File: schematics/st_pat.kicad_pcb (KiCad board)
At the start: 2 copper layers, 121.9 x 87 mm, 21 parts, among them J4 BATTERY, SW1 SW_PWR, SW2 BTN_RST, SW3 BTN, SW4 BTN, SW5 BTN, U1 GPS_Breakout_746, U2 FEATHER_M0_BASIC_PROTO, U3 LIS2MDL_ADAFRUIT, U4 Sharp_Display_4694, U5 COTS_GPS_RECEIVER, U6 SRAD_GPS_RECEIVER

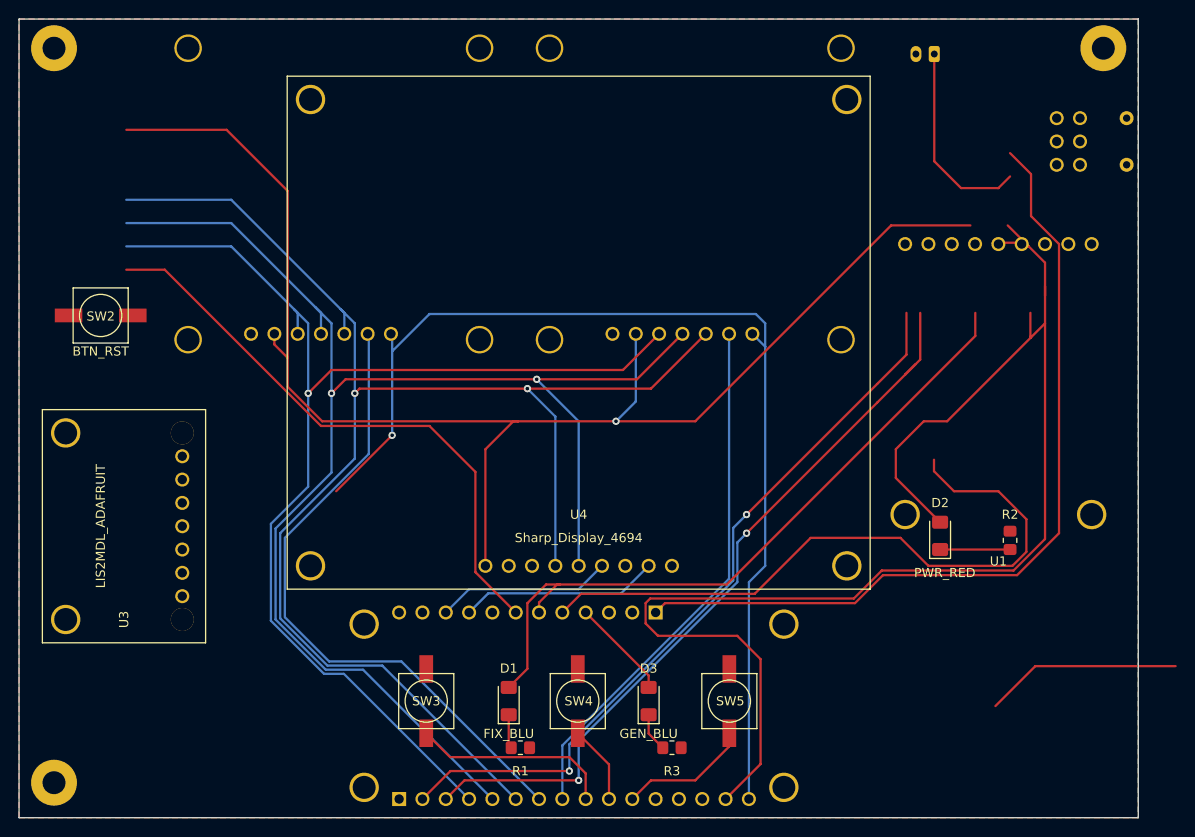
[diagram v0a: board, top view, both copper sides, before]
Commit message: wip: redo layout and use diffrent button footprint
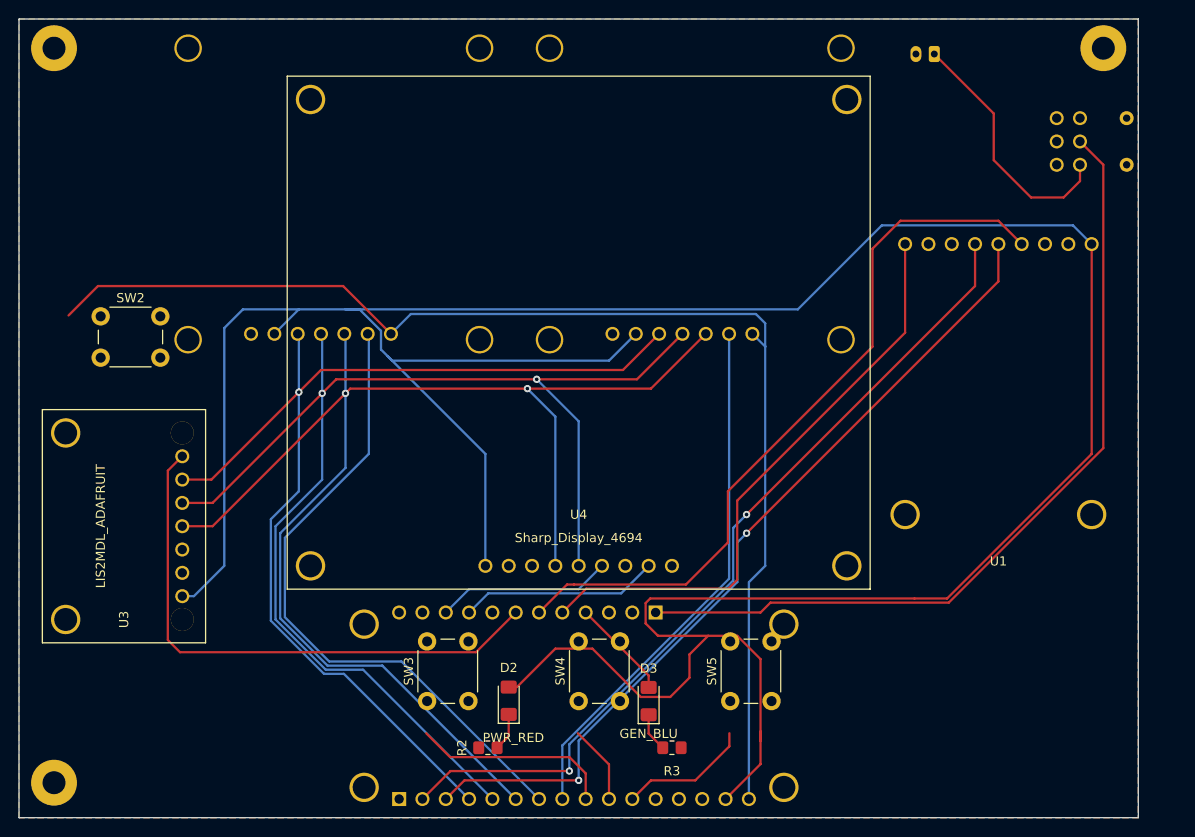
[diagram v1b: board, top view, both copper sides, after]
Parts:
- removed D1: FIX_BLU, LED_SMD:LED_1206_3216Metric_Pad1.42x1.75mm_HandSolder
- removed R1: 100, Resistor_SMD:R_0805_2012Metric_Pad1.20x1.40mm_HandSolder
- SW2, SW3, SW4, SW5: footprint st_pat:SW_Mini_Soft -> Button_Switch_THT:SW_PUSH_6mm
- moved R2 61.2 mm to (129.8, 116.8), turned to 180 degrees
- moved D2 50.3 mm to (132.1, 111.7)
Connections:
- SW1 pad 1: Net-(SW1-Pad1) -> (no net)
- SW1 pad 2: Net-(SW1-Pad2) -> (no net)
- SW1 pad 3: Net-(SW1-Pad3) -> (no net)
- SW1 pad 4: Net-(SW1-Pad4) -> (no net)
- U1 pad 2: Net-(U1-Pad2) -> (no net)
- U1 pad 7: Net-(U1-Pad7) -> (no net)
- U1 pad 8: Net-(U1-Pad8) -> (no net)
- U2 pad P1_12: Net-(U2-PadP1_12) -> (no net)
- U2 pad P1_14: Net-(U2-PadP1_14) -> (no net)
- U2 pad P2_11: Net-(U2-PadP2_11) -> (no net)
- U2 pad P2_12: Net-(U2-PadP2_12) -> (no net)
- U2 pad P2_2: Net-(U2-PadP2_2) -> (no net)
- U2 pad P2_3: Net-(U2-PadP2_3) -> (no net)
- U2 pad P2_8: Net-(U2-PadP2_8) -> (no net)
- U3 pad 2: Net-(U3-Pad2) -> (no net)
- U4 pad 2: Net-(U4-Pad2) -> (no net)
- U4 pad 7: Net-(U4-Pad7) -> (no net)
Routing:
- net +3V3: track 312.8 -> 341.4 mm, vias 1 -> 0
- net /GPS_RX: track 82.4 -> 93.0 mm
- net /MOSI: track 159.7 -> 149.5 mm
- net /SCK: track 164.1 -> 154.2 mm
- net /MISO: track 130.7 -> 120.9 mm
- net /GPS_TX: track 83.3 -> 92.7 mm
- net /GPS_PPS_D12: track 72.8 -> 64.7 mm
- net Net-(J4-Pad1): track 21.7 -> 27.8 mm
- net Net-(D1-Pad1): track 4.09 -> 0.00 mm
- net Net-(D2-Pad1): track 7.62 -> 4.16 mm
- net /CPS_CS_D10: track 64.3 -> 60.9 mm
- net /GPS_FIX_D11: track 77.6 -> 80.8 mm
- net /RST: track 138.4 -> 135.4 mm, vias 1 -> 0
